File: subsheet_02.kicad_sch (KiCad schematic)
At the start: 3 parts, among them J301 JTAG+VPP, U301 ATF1508AS_L_100A_TQFP_JTAG_EN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

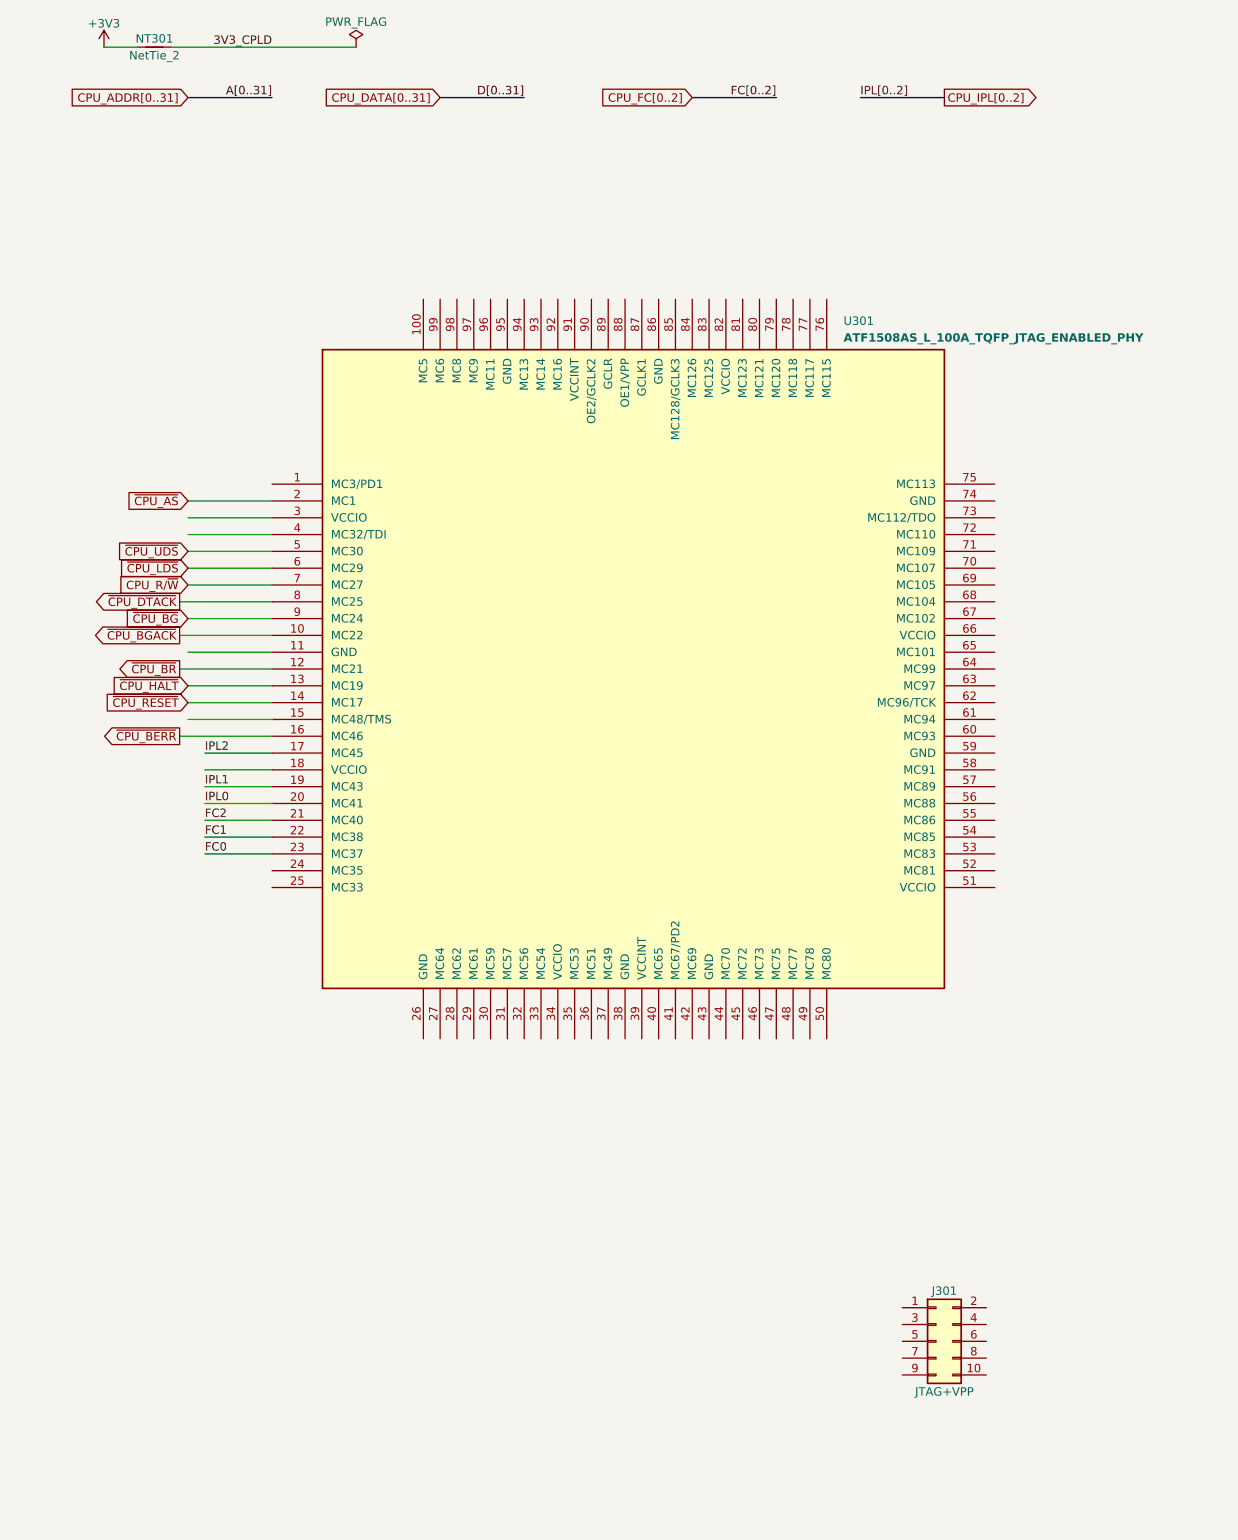
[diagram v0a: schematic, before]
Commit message: Continue CPLD
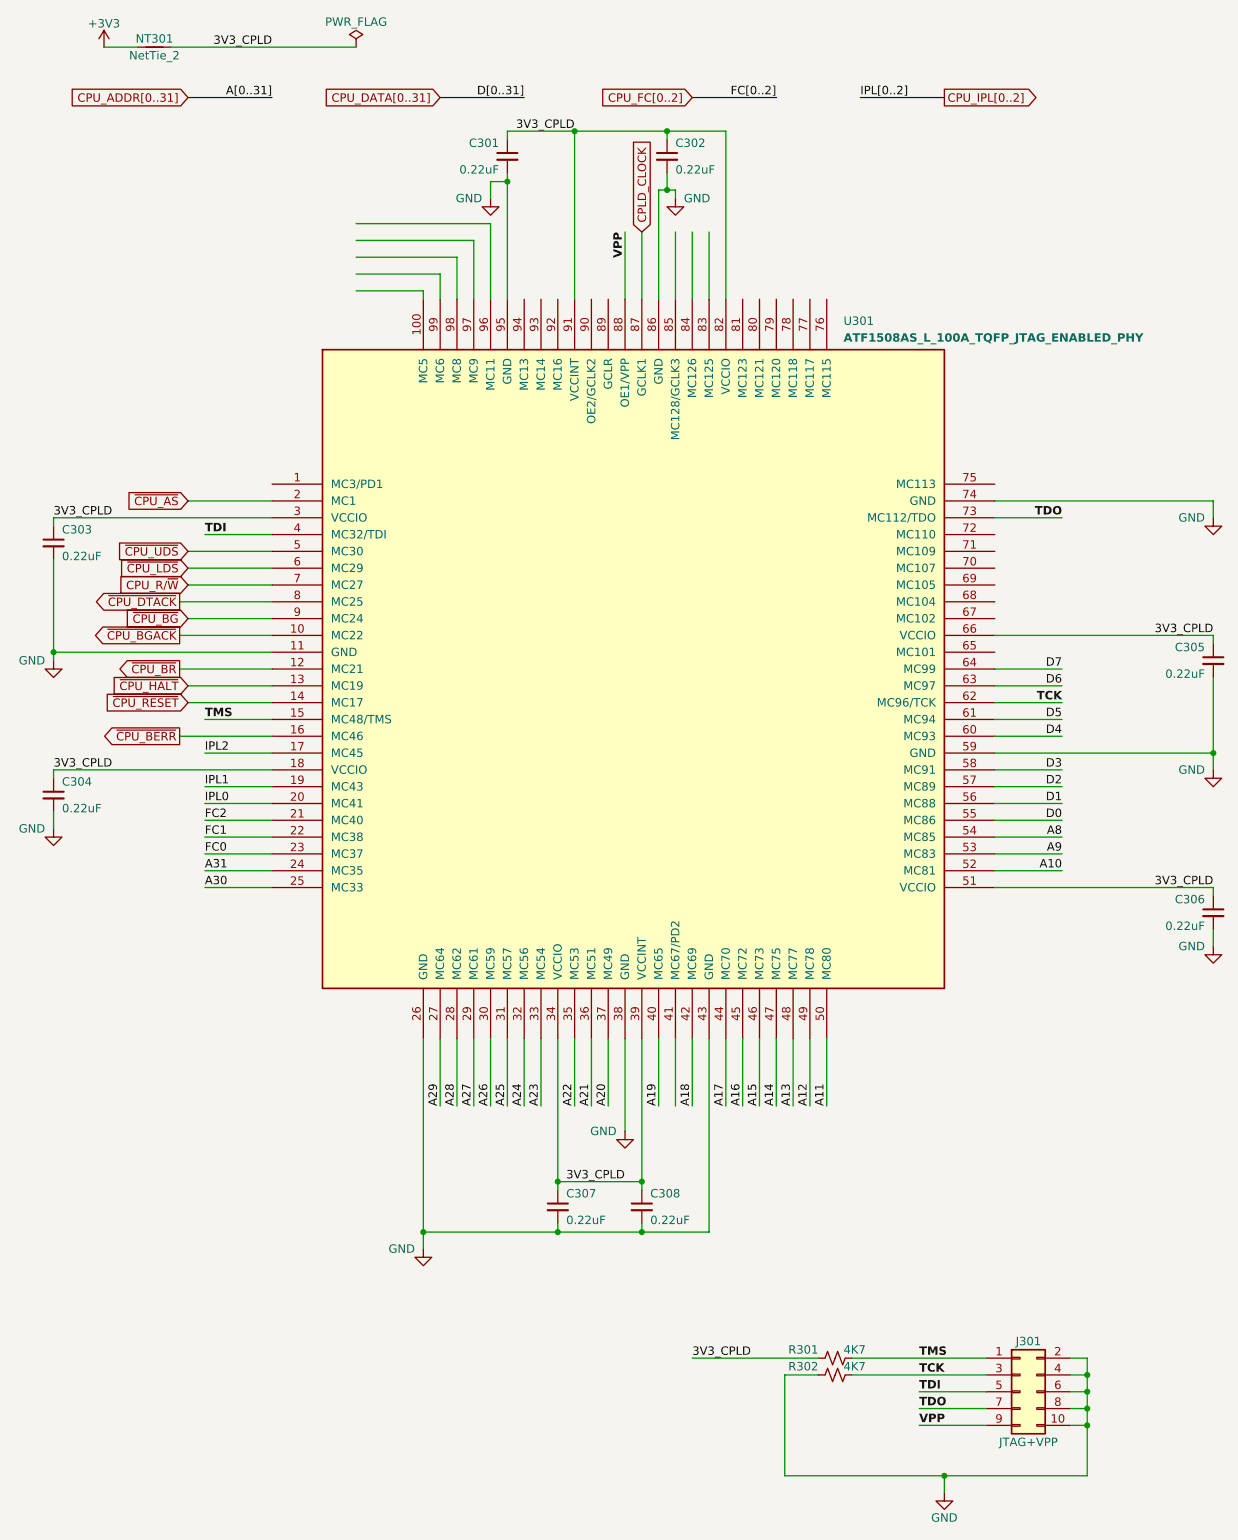
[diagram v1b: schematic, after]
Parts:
- added C301, C302, C303, C304, C305, C306, C307, C308: 0.22uF, symbol Device:C_Small
- added R301, R302: 4K7, symbol Device:R_Small_US
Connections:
- net 3V3_CPLD: now also U301.18 (VCCIO), U301.3 (VCCIO), U301.34 (VCCIO), U301.39 (VCCINT), U301.51 (VCCIO), U301.66 (VCCIO), U301.82 (VCCIO), U301.91 (VCCINT), C301.1, C302.1, C303.1, C304.1, C305.1, C306.1, C307.1, C308.1, R301.1
- net TMS: now reaches J301.1 (Pin_1)
- net TMS: now also U301.15 (MC48/TMS), R301.2
- net GND: now reaches J301.10 (Pin_10)
- net GND: now also J301.2 (Pin_2), J301.4 (Pin_4), J301.6 (Pin_6), J301.8 (Pin_8), U301.11 (GND), U301.26 (GND), U301.38 (GND), U301.43 (GND), U301.59 (GND), U301.74 (GND), U301.86 (GND), U301.95 (GND), C301.2, C302.2, C303.2, C304.2, C305.2, C306.2, C307.2, C308.2, R302.1
- net TCK: now reaches J301.3 (Pin_3)
- net TCK: now also U301.62 (MC96/TCK), R302.2
- net TDI: now reaches J301.5 (Pin_5)
- net TDI: now also U301.4 (MC32/TDI)
- net TDO: now reaches J301.7 (Pin_7)
- net TDO: now also U301.73 (MC112/TDO)
- net VPP: now reaches J301.9 (Pin_9)
- net VPP: now also U301.88 (OE1/VPP)
- net A31: now reaches U301.24 (MC35)
- net A30: now reaches U301.25 (MC33)
- net A29: now reaches U301.27 (MC64)
- net A28: now reaches U301.28 (MC62)
- net A27: now reaches U301.29 (MC61)
- net A26: now reaches U301.30 (MC59)
- net A25: now reaches U301.31 (MC57)
- net A24: now reaches U301.32 (MC56)
- net A23: now reaches U301.33 (MC54)
- net A22: now reaches U301.35 (MC53)
- net A21: now reaches U301.36 (MC51)
- net A20: now reaches U301.37 (MC49)
- net A19: now reaches U301.40 (MC65)
- net A18: now reaches U301.42 (MC69)
- net A17: now reaches U301.44 (MC70)
- net A16: now reaches U301.45 (MC72)
- net A15: now reaches U301.46 (MC73)
- net A14: now reaches U301.47 (MC75)
- net A13: now reaches U301.48 (MC77)
- net A12: now reaches U301.49 (MC78)
- net A11: now reaches U301.50 (MC80)
- net A10: now reaches U301.52 (MC81)
- net A9: now reaches U301.53 (MC83)
- net A8: now reaches U301.54 (MC85)
- net D0: now reaches U301.55 (MC86)
- net D1: now reaches U301.56 (MC88)
- net D2: now reaches U301.57 (MC89)
- net D3: now reaches U301.58 (MC91)
- net D4: now reaches U301.60 (MC93)
- net D5: now reaches U301.61 (MC94)
- net D6: now reaches U301.63 (MC97)
- net D7: now reaches U301.64 (MC99)
- net CPLD_CLOCK: now reaches U301.87 (GCLK1)
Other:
- moved on the sheet: J301
